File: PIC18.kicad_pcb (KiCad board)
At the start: 2 copper layers, 80 x 80 mm, 75 parts, among them J1 Conn_02x20_Odd_Even, J10 Port B, J11 Port C, J12 Port D, J13 Conn_01x03, J14 Conn_01x03, J15 Conn_01x03, J16 Conn_01x03, J2 Conn_01x06, J3 USB_A, J4 Conn_01x03, J5 Conn_01x02, J6 Conn_01x02, J7 USB_OTG, J8 Port A, J9 Port E, U1 PIC18F4620, U2 LM4040DBZ-4.1, U3 FT230XS, Y1 8 MHz

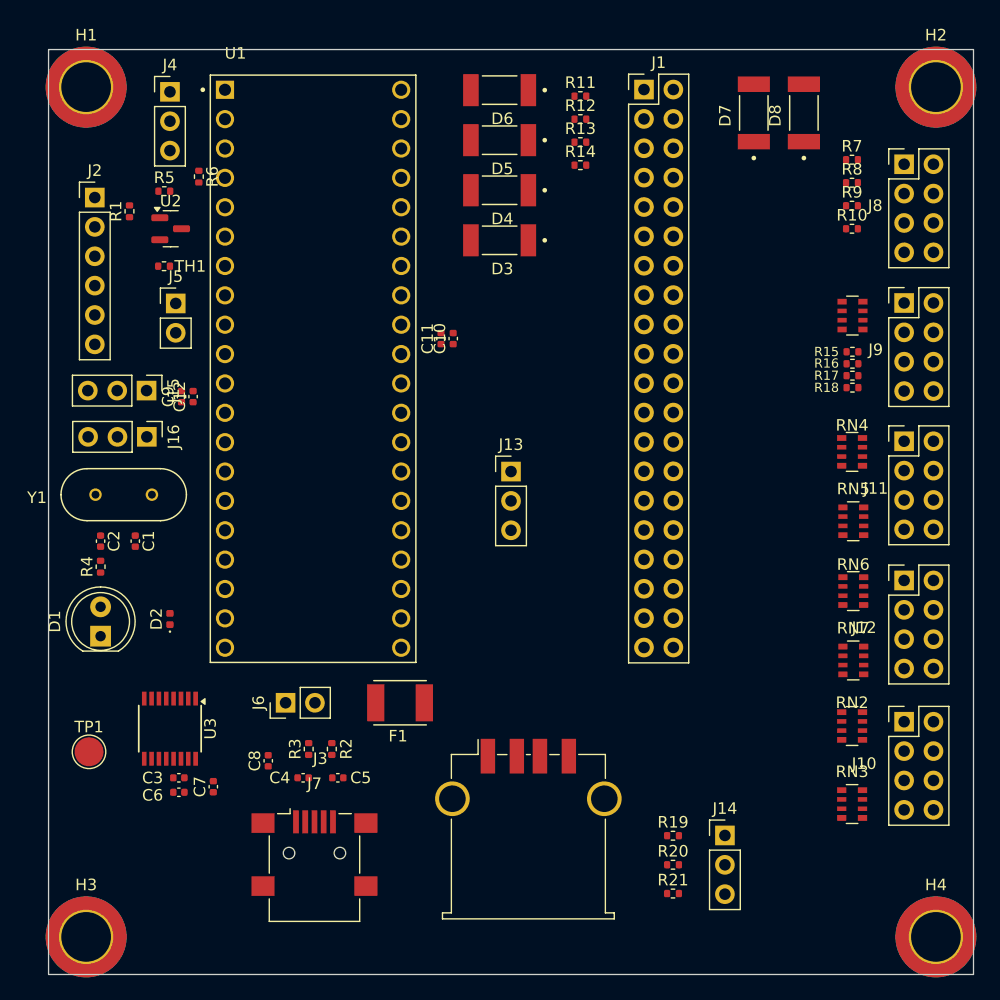
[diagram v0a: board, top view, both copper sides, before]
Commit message: Routing
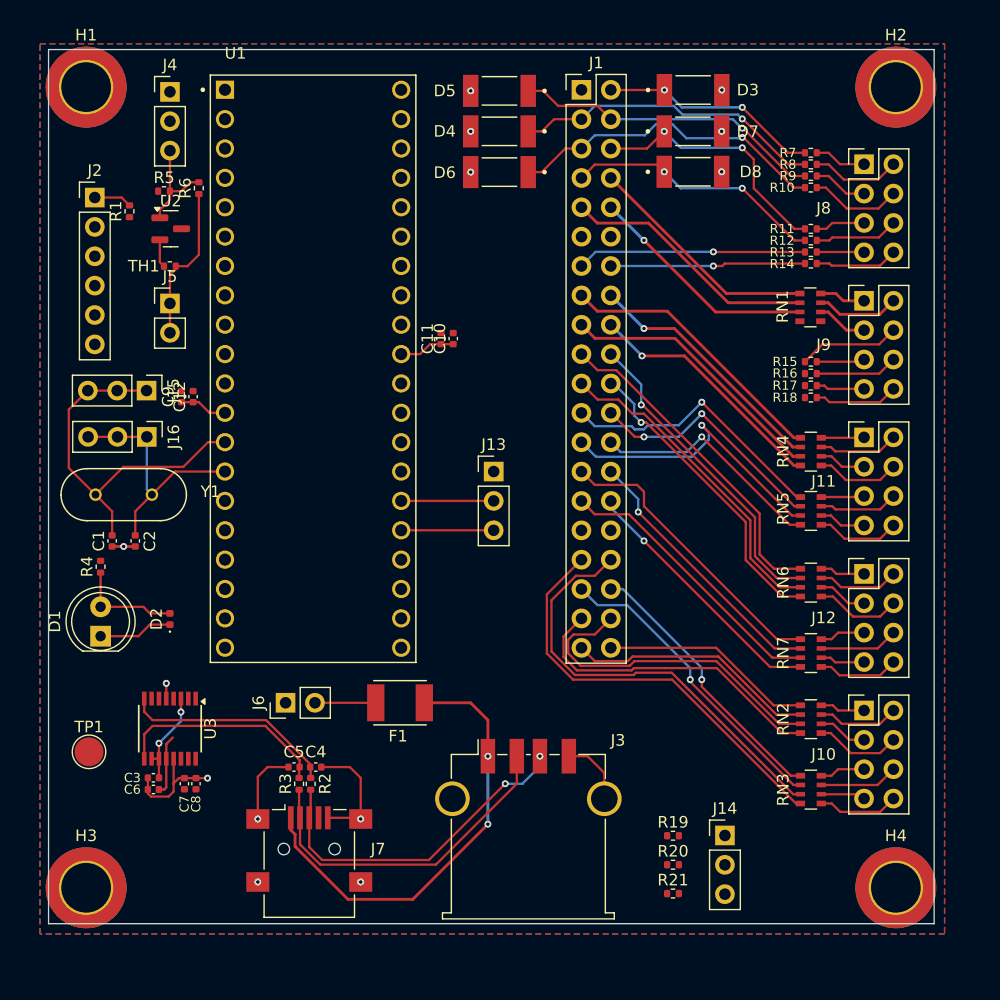
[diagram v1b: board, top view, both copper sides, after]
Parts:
- C6: value 100n -> 100nF
- moved R11 23.0 mm to (165.4, 81.0)
- moved R12 22.5 mm to (165.4, 82.0)
- moved R13 22.1 mm to (165.4, 83.0)
- moved R14 21.7 mm to (165.4, 84.0)
- moved D3 21.2 mm to (155.2, 69.0), turned to 0 degrees
- moved D8 10.9 mm to (155.2, 76.1), turned to 0 degrees
- moved D6 7.09 mm to (138.5, 76.1)
- moved C8 6.56 mm to (112.2, 129.0), turned to -90 degrees
- moved D7 5.50 mm to (155.2, 72.6), turned to 0 degrees
- moved H4 5.48 mm to (172.8, 138.0)
- moved J1 5.41 mm to (145.6, 69.0)
- moved D4 5.10 mm to (138.5, 72.6)
- moved R10 5.03 mm to (165.4, 77.4)
- moved R9 4.39 mm to (165.4, 76.4)
- moved D5 4.27 mm to (138.5, 69.1)
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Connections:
- J13 pad 1: unconnected-(J13-Pin_1-Pad1) -> GND
- J4 pad 2: /RA1/AN1 -> /VREF+
- J4 pad 3: /RA3/AN3/VREF+ -> Net-(J4-Pin_3)
- J7 pad 1: VCC -> Net-(J3-VBUS)
- J9 pad 4: /RA3/AN3/VREF+ -> /VREF+
- R15 pad 1: /RA3/AN3/VREF+ -> /VREF+
- R16 pad 1: /RA3/AN3/VREF+ -> /VREF+
- R17 pad 1: /RA3/AN3/VREF+ -> /VREF+
- R18 pad 1: /RA3/AN3/VREF+ -> /VREF+
- R5 pad 2: /RA3/AN3/VREF+ -> Net-(J4-Pin_3)
- R6 pad 2: /RA3/AN3/VREF+ -> Net-(J4-Pin_3)
- U2 pad 1: /RA3/AN3/VREF+ -> Net-(J4-Pin_3)
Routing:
- net GND: track 0.00 -> 53.8 mm, vias 0 -> 13
- net /OSC1/CLKI/RA7: track 0.00 -> 52.8 mm, vias 0 -> 1
- net Net-(J3-VBUS): track 0.00 -> 39.0 mm, vias 0 -> 2
- net /OSC2/CLKO/RA6: track 0.00 -> 38.4 mm, vias 0 -> 1
- net /RB1/INT1/AN10: track 0.00 -> 37.8 mm
- net /RB0/INT0/FLT0/AN12: track 0.00 -> 36.7 mm
- net /RC6/TX/CK: track 0.00 -> 33.4 mm, vias 0 -> 1
- net Net-(J3-D+): track 0.00 -> 29.7 mm, vias 0 -> 2
- net Net-(J3-D-): track 0.00 -> 29.5 mm
- net /RD0/PSP0: track 0.00 -> 28.7 mm
- net /RB5/KBI1/PGM: track 0.00 -> 28.6 mm
- net /RC7/RX/DT: track 0.00 -> 28.4 mm, vias 0 -> 1
- net /RD2/PSP2: track 0.00 -> 28.2 mm
- net /RA3/AN3/VREF+: track 0.00 -> 28.0 mm, vias 0 -> 1
- net /RD1/PSP1: track 0.00 -> 27.4 mm, vias 0 -> 1
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- added copper zone on B.Cu, net GND
- added copper zone on F.Cu, net VCC
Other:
- board size 80 x 80 mm -> 76.6 x 75.6 mm
